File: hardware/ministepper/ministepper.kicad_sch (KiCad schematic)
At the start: 9 parts, among them U1 STM32G071G8U6, U4 SIT3088EEUA

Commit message: ministepper: add (justify left/right) to hier labels and sheet pins
The labels inside stepper_channel.kicad_sch and the sheet-block pins
on the root ministepper.kicad_sch were missing (justify ...) inside
their (effects ...) — which left KiCad to render the text with no
offset from the arrow glyph. User caught it by hand-placing a FOO
hier label in KiCad which came out formatted with (justify left).

Fixed 13 hier labels in the sub-sheet and 24 pins across the two
stepper sheet instances on the root:

  angle 0   (left edge on sub-sheet, or right edge on root sheet) -> justify left
  angle 180 (right edge on sub-sheet, or left edge on root sheet) -> justify right

Text now sits cleanly on the INSIDE side of each pin's triangle glyph
with the standard KiCad offset instead of overlapping the first
letter of each label.
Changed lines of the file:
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@@
 		(at 48.26 100)
 		(size 40 30)
+		(exclude_from_sim no)
+		(in_bom yes)
+		(on_board yes)
+		(dnp no)
 		(fields_autoplaced yes)
-		(stroke (width 0.1524) (type solid))
-		(fill (color 225 240 255 1))
+		(stroke
+			(width 0.1524)
+			(type solid)
+		)
+		(fill
+			(color 225 240 255 1)
+		)
 		(property "Sheetname" "Stepper 1"
 			(at 48.26 99.2884 0)
-			(effects (font (size 1.27 1.27)) (justify left bottom))
+			(show_name no)
+			(do_not_autoplace no)
+			(effects
+				(font
+					(size 1.27 1.27)
+				)
+				(justify left bottom)
+			)
 		)
 		(property "Sheetfile" "stepper_channel.kicad_sch"
 			(at 48.26 130.8146 0)
-			(effects (font (size 1.27 1.27)) (justify left top))
+			(show_name no)
+			(do_not_autoplace no)
+			(effects
+				(font
+					(size 1.27 1.27)
+				)
+				(justify left top)
+			)
 		)
 		(pin "SCK" input
 			(at 48.26 102.54 180)
-			(effects (font (size 1.27 1.27)) (justify left))
+			(effects
+				(font
+					(size 1.27 1.27)
+				)
+			)
 		)
 		(pin "MOSI" input
-			(at 48.26 105.08000000000001 180)
-			(effects (font (size 1.27 1.27)) (justify left))
+			(at 48.26 105.08 180)
+			(effects
+				(font
+					(size 1.27 1.27)
+				)
+			)
 		)
 		(pin "MISO" output
 			(at 48.26 107.62 180)
-			(effects (font (size 1.27 1.27)) (justify left))
+			(effects
+				(font
+					(size 1.27 1.27)
+				)
+			)
 		)
 		(pin "CS" input
-			(at 48.26 110.16000000000001 180)
-			(effects (font (size 1.27 1.27)) (justify left))
+			(at 48.26 110.16 180)
+			(effects
+				(font
+					(size 1.27 1.27)
+				)
+			)
 		)
 		(pin "STEP" input
 			(at 48.26 112.7 180)
-			(effects (font (size 1.27 1.27)) (justify left))
+			(effects
+				(font
+					(size 1.27 1.27)
+				)
+			)
 		)
 		(pin "DIR" input
-			(at 48.26 115.24000000000001 180)
-			(effects (font (size 1.27 1.27)) (justify left))
+			(at 48.26 115.24 180)
+			(effects
+				(font
+					(size 1.27 1.27)
+				)
+			)
 		)
 		(pin "DRV_ENN" input
 			(at 48.26 117.78 180)
-			(effects (font (size 1.27 1.27)) (justify left))
+			(effects
+				(font
+					(size 1.27 1.27)
+				)
+			)
 		)
 		(pin "DIAG1" output
-			(at 48.26 120.32000000000001 180)
-			(effects (font (size 1.27 1.27)) (justify left))
+			(at 48.26 120.32 180)
+			(effects
+				(font
+					(size 1.27 1.27)
+				)
+			)
 		)
 		(pin "MOT_A+" output
-			(at 88.25999999999999 102.54 0)
-			(effects (font (size 1.27 1.27)) (justify right))
+			(at 88.26 102.54 0)
+			(effects
+				(font
+					(size 1.27 1.27)
+				)
+			)
 		)
 		(pin "MOT_A-" output
-			(at 88.25999999999999 105.08000000000001 0)
-			(effects (font (size 1.27 1.27)) (justify right))
+			(at 88.26 105.08 0)
+			(effects
+				(font
+					(size 1.27 1.27)
+				)
+			)
 		)
 		(pin "MOT_B+" output
-			(at 88.25999999999999 107.62 0)
-			(effects (font (size 1.27 1.27)) (justify right))
+			(at 88.26 107.62 0)
+			(effects
+				(font
+					(size 1.27 1.27)
+				)
+			)
 		)
 		(pin "MOT_B-" output
-			(at 88.25999999999999 110.16000000000001 0)
-			(effects (font (size 1.27 1.27)) (justify right))
+			(at 88.26 110.16 0)
+			(effects
+				(font
+					(size 1.27 1.27)
+				)
+			)
 		)
 	)
@@
 		(at 101.6 100)
 		(size 40 30)
+		(exclude_from_sim no)
+		(in_bom yes)
+		(on_board yes)
+		(dnp no)
 		(fields_autoplaced yes)
-		(stroke (width 0.1524) (type solid))
-		(fill (color 225 255 225 1))
+		(stroke
+			(width 0.1524)
+			(type solid)
+		)
+		(fill
+			(color 225 255 225 1)
+		)
 		(property "Sheetname" "Stepper 2"
 			(at 101.6 99.2884 0)
-			(effects (font (size 1.27 1.27)) (justify left bottom))
+			(show_name no)
+			(do_not_autoplace no)
+			(effects
+				(font
+					(size 1.27 1.27)
+				)
+				(justify left bottom)
+			)
 		)
 		(property "Sheetfile" "stepper_channel.kicad_sch"
 			(at 101.6 130.8146 0)
-			(effects (font (size 1.27 1.27)) (justify left top))
+			(show_name no)
+			(do_not_autoplace no)
+			(effects
+				(font
+					(size 1.27 1.27)
+				)
+				(justify left top)
+			)
 		)
 		(pin "SCK" input
 			(at 101.6 102.54 180)
-			(effects (font (size 1.27 1.27)) (justify left))
+			(effects
+				(font
+					(size 1.27 1.27)
+				)
+			)
 		)
 		(pin "MOSI" input
-			(at 101.6 105.08000000000001 180)
-			(effects (font (size 1.27 1.27)) (justify left))
+			(at 101.6 105.08 180)
+			(effects
+				(font
+					(size 1.27 1.27)
+				)
+			)
 		)
 		(pin "MISO" output
 			(at 101.6 107.62 180)
-			(effects (font (size 1.27 1.27)) (justify left))
+			(effects
+				(font
+					(size 1.27 1.27)
+				)
+			)
 		)
 		(pin "CS" input
-			(at 101.6 110.16000000000001 180)
-			(effects (font (size 1.27 1.27)) (justify left))
+			(at 101.6 110.16 180)
+			(effects
+				(font
+					(size 1.27 1.27)
+				)
+			)
 		)
 		(pin "STEP" input
 			(at 101.6 112.7 180)
-			(effects (font (size 1.27 1.27)) (justify left))
+			(effects
+				(font
+					(size 1.27 1.27)
+				)
+			)
 		)
 		(pin "DIR" input
-			(at 101.6 115.24000000000001 180)
-			(effects (font (size 1.27 1.27)) (justify left))
+			(at 101.6 115.24 180)
+			(effects
+				(font
+					(size 1.27 1.27)
+				)
+			)
 		)
 		(pin "DRV_ENN" input
 			(at 101.6 117.78 180)
-			(effects (font (size 1.27 1.27)) (justify left))
+			(effects
+				(font
+					(size 1.27 1.27)
+				)
+			)
 		)
 		(pin "DIAG1" output
-			(at 101.6 120.32000000000001 180)
-			(effects (font (size 1.27 1.27)) (justify left))
+			(at 101.6 120.32 180)
+			(effects
+				(font
+					(size 1.27 1.27)
+				)
+			)
 		)
 		(pin "MOT_A+" output
 			(at 141.6 102.54 0)
-			(effects (font (size 1.27 1.27)) (justify right))
+			(effects
+				(font
+					(size 1.27 1.27)
+				)
+			)
 		)
 		(pin "MOT_A-" output
-			(at 141.6 105.08000000000001 0)
-			(effects (font (size 1.27 1.27)) (justify right))
+			(at 141.6 105.08 0)
+			(effects
+				(font
+					(size 1.27 1.27)
+				)
+			)
 		)
 		(pin "MOT_B+" output
 			(at 141.6 107.62 0)
-			(effects (font (size 1.27 1.27)) (justify right))
+			(effects
+				(font
+					(size 1.27 1.27)
+				)
+			)
 		)
 		(pin "MOT_B-" output
-			(at 141.6 110.16000000000001 0)
-			(effects (font (size 1.27 1.27)) (justify right))
+			(at 141.6 110.16 0)
+			(effects
+				(font
+					(size 1.27 1.27)
+				)
+			)
 		)
 	)

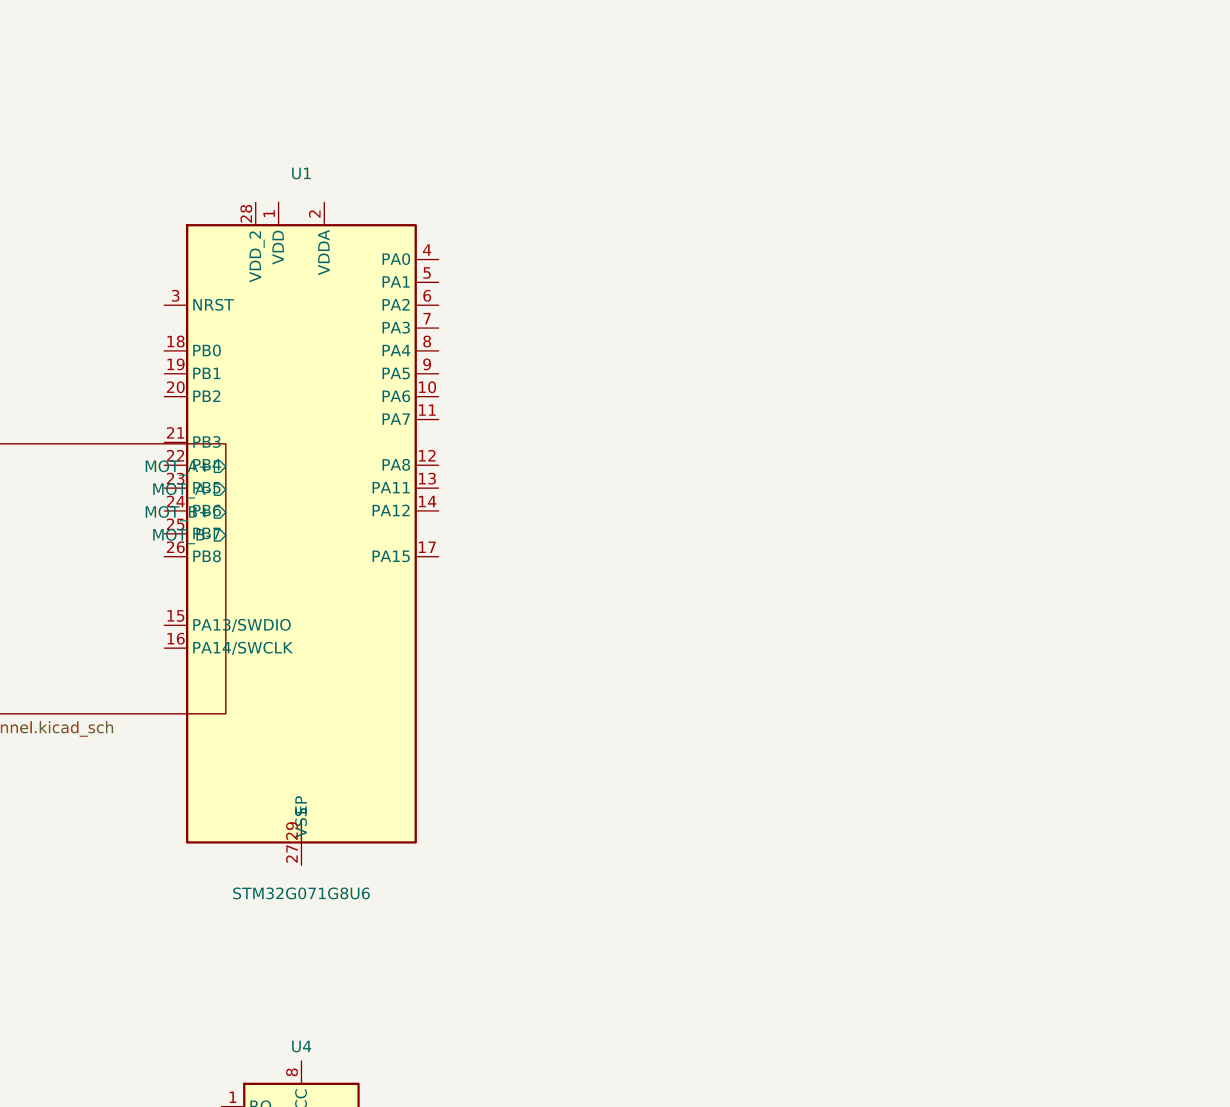
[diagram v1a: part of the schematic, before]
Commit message: pcb
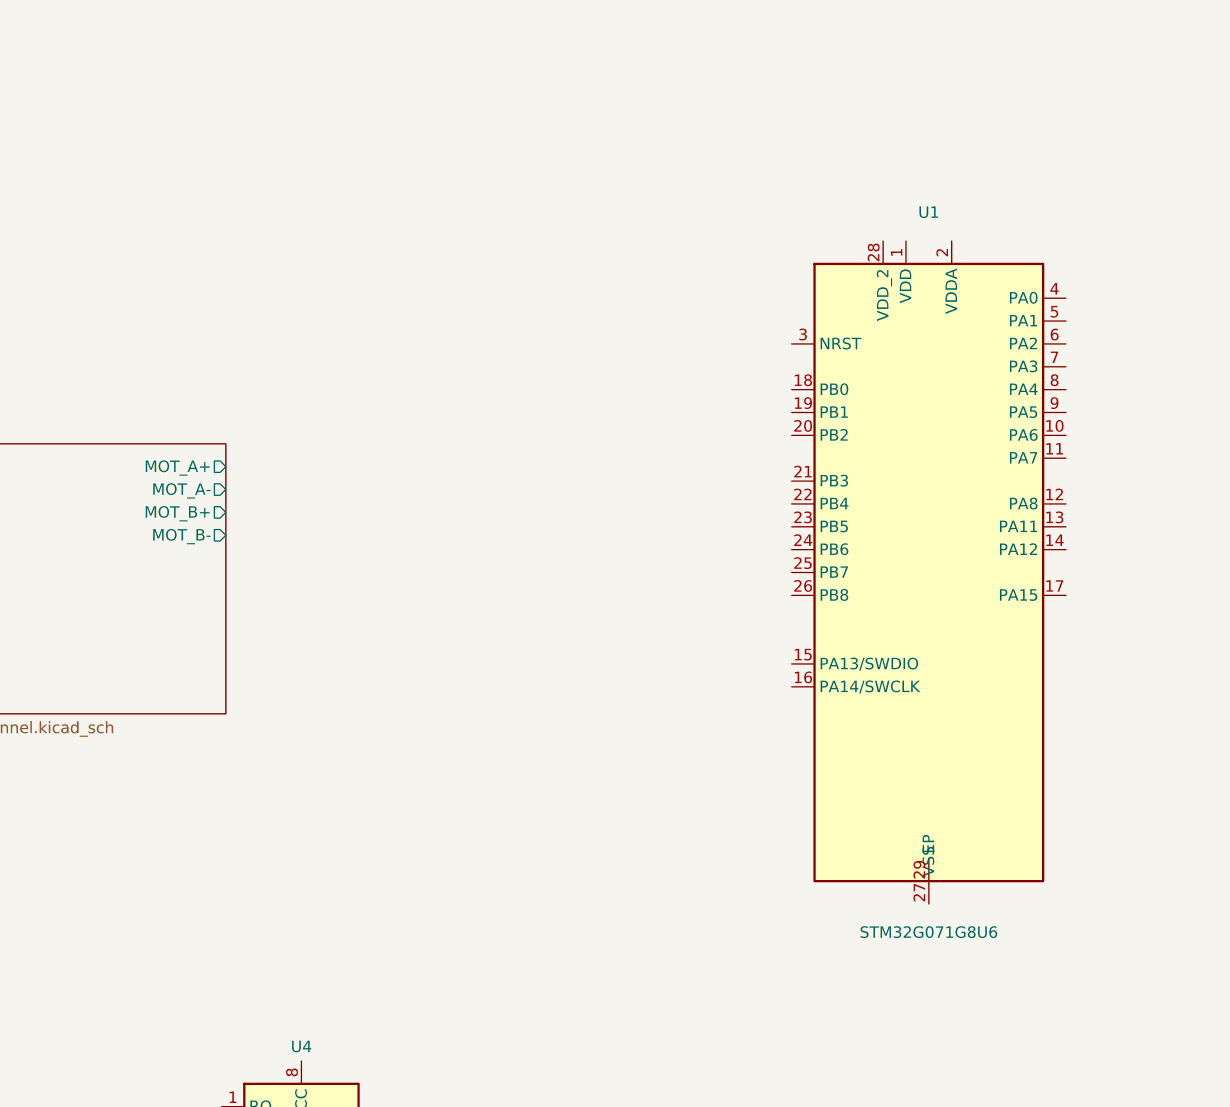
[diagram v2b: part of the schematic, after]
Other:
- moved on the sheet: U1
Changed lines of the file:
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@@
 	(symbol
 		(lib_id "tsumikoro:STM32G071G8U6")
-		(at 150 110 0)
+		(at 219.71 114.3 0)
 		(unit 1)
 		(body_style 1)
@@
 		(dnp no)
 		(property "Reference" "U1"
-			(at 150 70 0)
+			(at 219.71 74.3 0)
 			(show_name no)
 			(do_not_autoplace no)
@@
 		)
 		(property "Value" "STM32G071G8U6"
-			(at 150 150 0)
+			(at 219.71 154.3 0)
 			(show_name no)
 			(do_not_autoplace no)
@@
 		)
 		(property "Footprint" "tsumikoro:UFQFPN-28"
-			(at 150 110 0)
+			(at 219.71 114.3 0)
 			(hide yes)
 			(show_name no)
@@
 		)
 		(property "Datasheet" "https://www.st.com/resource/en/datasheet/stm32g071g8.pdf"
-			(at 150 110 0)
+			(at 219.71 114.3 0)
 			(hide yes)
 			(show_name no)
@@
 		)
 		(property "Description" "ARM Cortex-M0+ 64MHz, 64KB Flash, 36KB RAM, UFQFPN-28"
-			(at 150 110 0)
+			(at 219.71 114.3 0)
 			(hide yes)
 			(show_name no)
@@
 		)
 		(property "LCSC" "C724080"
-			(at 150 110 0)
+			(at 219.71 114.3 0)
 			(hide yes)
 			(show_name no)
@@
 		)
 		(property "MPN" "STM32G071G8U6"
-			(at 150 110 0)
+			(at 219.71 114.3 0)
 			(hide yes)
 			(show_name no)
@@
 		)
 		(property "Manufacturer" "STMicroelectronics"
-			(at 150 110 0)
+			(at 219.71 114.3 0)
 			(hide yes)
 			(show_name no)
